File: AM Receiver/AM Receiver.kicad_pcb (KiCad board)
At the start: 2 copper layers, 88.8 x 40.2 mm, 74 parts, among them IC1 NE612AD, IC2 NE612AD, IC3 74HC74, IC4 TDA1072AT, IC5 74HTC4046, IC7 L78L05_SO8, P1 10k, P2 50k, P3 50k, Q1 MMBFJ310LT1G, Q2 MMBFJ310LT1G, Q3 BC547, Q4 BC547, Q5 BC557, U6 L78L08_SO8

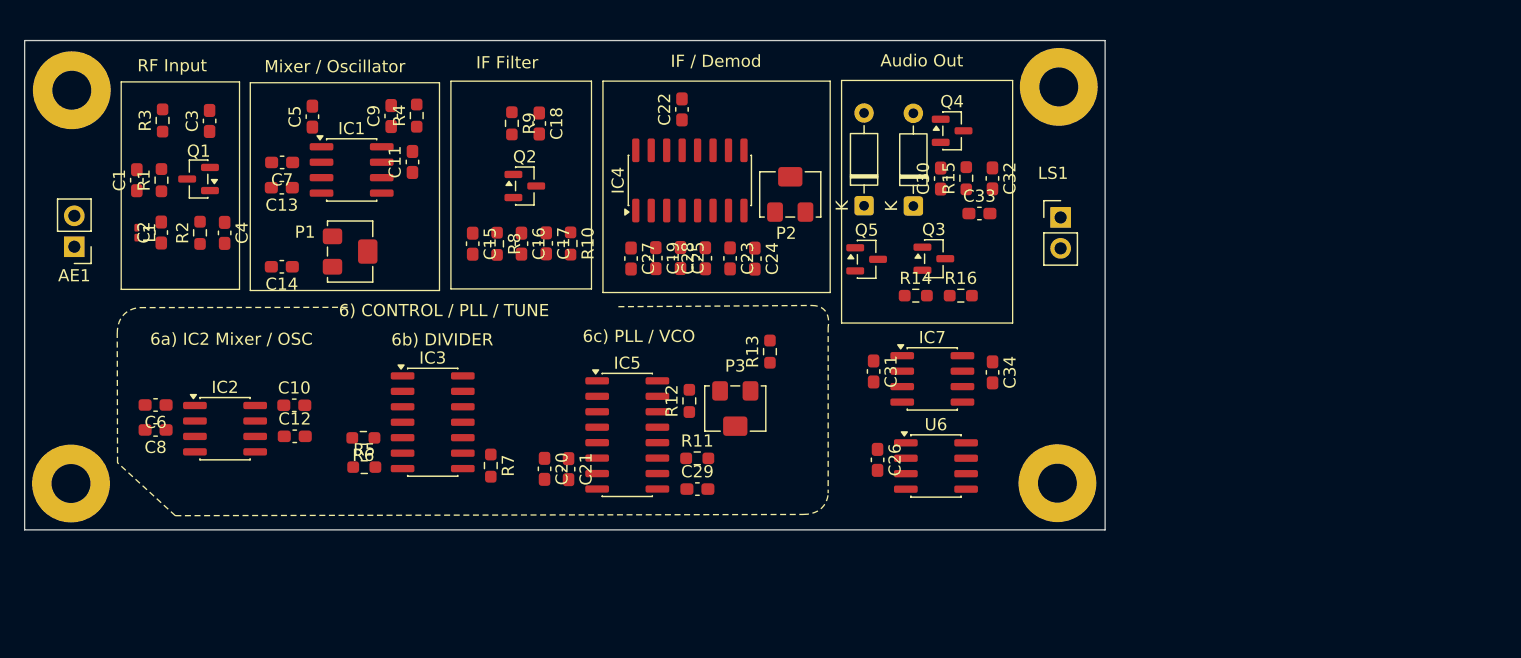
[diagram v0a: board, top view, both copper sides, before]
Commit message: Finished PCB design for AM Receiver and fixed all remaining errors
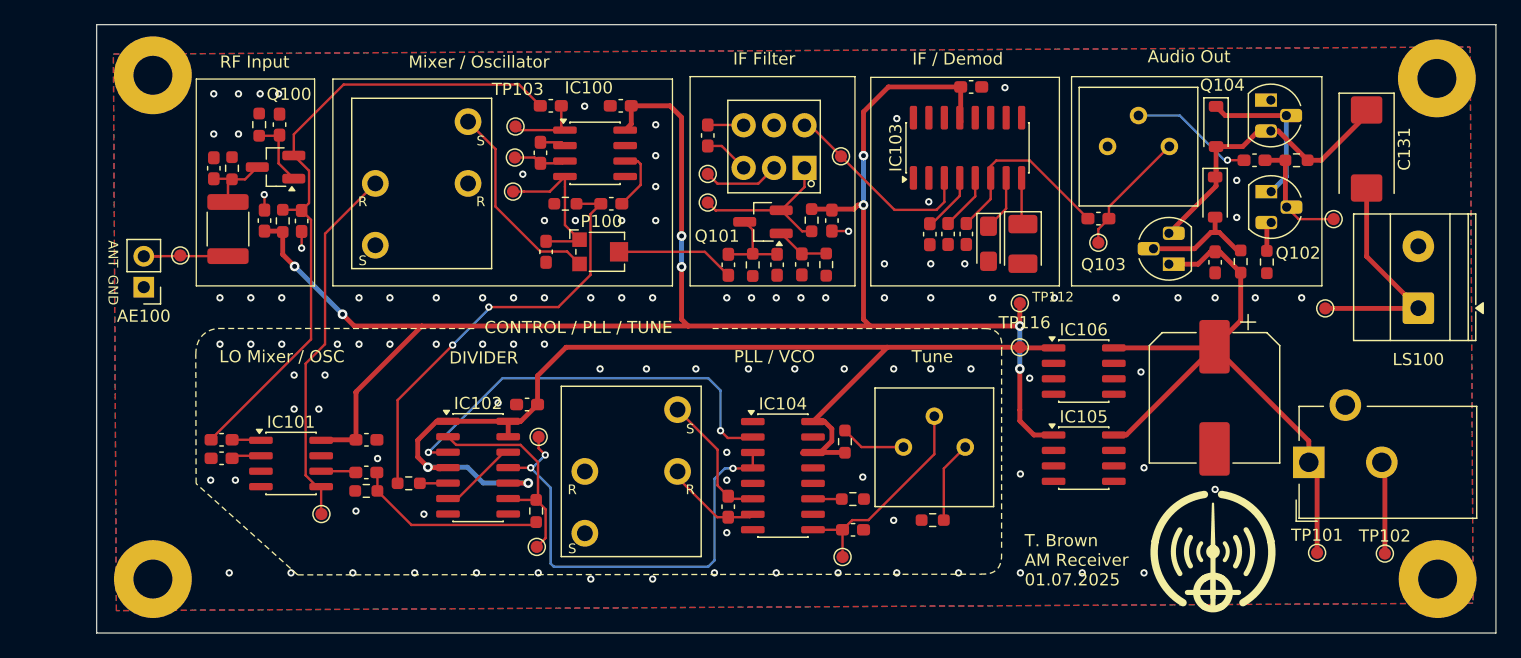
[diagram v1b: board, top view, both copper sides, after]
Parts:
- added AM_Radio_Logo: , AM_Radio:AM_Radio_logo, F.Cu at (184.2, 114.7)
- added FL100: SFZ455A, AM_Radio:SFZ455A, F.Cu at (148.2, 81.2)
- added J100: Barrel_Jack_Switch, Connector_BarrelJack:BarrelJack_CUI_PJ-102AH_Horizontal, F.Cu at (192.2, 107.2)
- added TP100: ANT_IN, TestPoint:TestPoint_Pad_D1.0mm, F.Cu at (99.4, 90.2)
- added TP101: TP_VIN, TestPoint:TestPoint_Pad_D1.0mm, F.Cu at (192.8, 114.6)
- added TP102: TP_GND, TestPoint:TestPoint_Pad_D1.0mm, F.Cu at (198.4, 114.7)
- added TP103: TP_MIXER_IN, TestPoint:TestPoint_Pad_D1.0mm, F.Cu at (127.0, 79.6)
- added TP104: TP_GND_RF, TestPoint:TestPoint_Pad_D1.0mm, F.Cu at (126.9, 82.1)
- added TP105: TP_RF_MIXER_OUT, TestPoint:TestPoint_Pad_D1.0mm, F.Cu at (126.8, 84.9)
- added TP106: TP_LO_MIXER_OUT, TestPoint:TestPoint_Pad_D1.0mm, F.Cu at (111.0, 111.4)
- added TP107: TP_IF_FILTER_IN, TestPoint:TestPoint_Pad_D1.0mm, F.Cu at (142.8, 85.8)
- added TP108: TP_DIV_OUT, TestPoint:TestPoint_Pad_D1.0mm, F.Cu at (128.7, 114.1)
- added TP109: TP_GND_IF, TestPoint:TestPoint_Pad_D1.0mm, F.Cu at (142.8, 83.5)
- added TP110: TP_IF_FILTER_OUT, TestPoint:TestPoint_Pad_D1.0mm, F.Cu at (153.7, 82.0)
- added TP111: TP_VCO_OUT, TestPoint:TestPoint_Pad_D1.0mm, F.Cu at (128.9, 105.1)
- added TP112: TP_8V, TestPoint:TestPoint_Pad_D1.0mm, F.Cu at (168.4, 94.1)
- added TP113: TP_AUDIO_DEMOD, TestPoint:TestPoint_Pad_D1.0mm, F.Cu at (174.9, 89.1)
- added TP114: TP_VCO_CTRL, TestPoint:TestPoint_Pad_D1.0mm, F.Cu at (153.8, 115.0)
- added TP115: TP_AUDIO_DRV, TestPoint:TestPoint_Pad_D1.0mm, F.Cu at (194.2, 87.2)
- added TP116: TP_5V, TestPoint:TestPoint_Pad_D1.0mm, F.Cu at (168.4, 97.7)
- added TP117: TP_SPK_OUT, TestPoint:TestPoint_Pad_D1.0mm, F.Cu at (193.5, 94.5)
- C113: renamed from C14; value 100p -> 7–100p; footprint Capacitor_SMD:C_0603_1608Metric_Pad1.08x0.95mm_HandSolder -> AM_Radio:Vishay_BFC280907015_Trimmer_7-100pF
- C120: renamed from C21; value 100p -> 7–100p; footprint Capacitor_SMD:C_0603_1608Metric_Pad1.08x0.95mm_HandSolder -> AM_Radio:Vishay_BFC280907015_Trimmer_7-100pF
- C122: renamed from C23; footprint Capacitor_SMD:C_0603_1608Metric_Pad1.08x0.95mm_HandSolder -> Capacitor_Tantalum_SMD:CP_EIA-3216-18_Kemet-A_HandSolder
- C123: renamed from C24; footprint Capacitor_SMD:C_0603_1608Metric_Pad1.08x0.95mm_HandSolder -> Capacitor_Tantalum_SMD:CP_EIA-3528-21_Kemet-B_HandSolder
- C131: renamed from C32; footprint Capacitor_SMD:C_0603_1608Metric_Pad1.08x0.95mm_HandSolder -> Capacitor_Tantalum_SMD:CP_EIA-7343-20_Kemet-V_HandSolder
- C132: renamed from C33; footprint Capacitor_SMD:C_0603_1608Metric_Pad1.08x0.95mm_HandSolder -> Capacitor_SMD:CP_Elec_10x10.5
- D100: renamed from D1; footprint Diode_THT:D_DO-35_SOD27_P7.62mm_Horizontal -> Diode_SMD:D_SOD-123
- D101: renamed from D2; footprint Diode_THT:D_DO-35_SOD27_P7.62mm_Horizontal -> Diode_SMD:D_SOD-123
- IC100: renamed from IC1; value NE612AD -> SA612AD
- IC101: renamed from IC2; value NE612AD -> SA612AD
- IC102: renamed from IC3; value 74HC74 -> 74HC74D
- IC104: renamed from IC5; value 74HTC4046 -> 74HCT4046AD
- L100: renamed from L1; footprint Inductor_SMD:L_0201_0603Metric_Pad0.64x0.40mm_HandSolder -> Inductor_SMD:L_1812_4532Metric_Pad1.30x3.40mm_HandSolder
- LS100: renamed from LS1; footprint Connector_PinHeader_2.54mm:PinHeader_1x02_P2.54mm_Vertical -> TerminalBlock_Phoenix:TerminalBlock_Phoenix_MKDS-1,5-2-5.08_1x02_P5.08mm_Horizontal
- P100: renamed from P1; footprint Potentiometer_SMD:Potentiometer_Bourns_3224W_Vertical -> Potentiometer_SMD:Potentiometer_Bourns_TC33X_Vertical
- P101: renamed from P2; footprint Potentiometer_SMD:Potentiometer_Bourns_3224W_Vertical -> Potentiometer_THT:Potentiometer_Bourns_3386P_Vertical
- P102: renamed from P3; footprint Potentiometer_SMD:Potentiometer_Bourns_3224W_Vertical -> Potentiometer_THT:Potentiometer_Bourns_3386P_Vertical
- Q100: renamed from Q1; value MMBFJ310LT1G -> MMBFJ310LT3G; footprint Package_TO_SOT_SMD:SOT-23 -> Package_TO_SOT_SMD:SOT-23_Handsoldering
- Q101: renamed from Q2; value MMBFJ310LT1G -> MMBFJ310LT3G; footprint Package_TO_SOT_SMD:SOT-23 -> Package_TO_SOT_SMD:SOT-23_Handsoldering
- Q102: renamed from Q3; footprint Package_TO_SOT_SMD:SOT-23 -> Package_TO_SOT_THT:TO-92_HandSolder
- Q103: renamed from Q4; footprint Package_TO_SOT_SMD:SOT-23 -> Package_TO_SOT_THT:TO-92_HandSolder
- Q104: renamed from Q5; footprint Package_TO_SOT_SMD:SOT-23 -> Package_TO_SOT_THT:TO-92_HandSolder
- moved Q104 35.7 mm to (189.0, 77.4), turned to -90 degrees
- moved R113 33.2 mm to (191.1, 82.4), turned to 180 degrees
- moved C127 32.5 mm to (174.9, 87.2), turned to 180 degrees
- moved H101 32.2 mm to (202.7, 116.8)
- moved P101 31.4 mm to (180.7, 81.2), turned to 90 degrees
- moved H102 31.1 mm to (202.7, 75.6)
- moved C131 30.8 mm to (196.9, 81.4)
- moved LS100 30.3 mm to (201.2, 94.5), turned to 90 degrees
- moved D101 29.7 mm to (184.5, 79.6), turned to -90 degrees
- moved C130 28.6 mm to (127.9, 102.4), turned to 180 degrees
- moved Q102 28.3 mm to (189.1, 84.9), turned to -90 degrees
- moved C126 27.6 mm to (164.0, 88.4)
- moved R108 25.9 mm to (151.3, 87.3)
- moved C129 25.8 mm to (187.7, 82.4), turned to 180 degrees
- moved R115 25.3 mm to (188.7, 90.7), turned to -90 degrees
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- renumbered AE1 to AE100, C1 to C100, C2 to C101, C3 to C102, C4 to C103, C5 to C104, C6 to C105, C7 to C106, C8 to C107, C9 to C108, C10 to C109, C11 to C110, C12 to C111, C13 to C112, C15 to C114, C16 to C115, C17 to C116, C18 to C117, C19 to C118, C20 to C119, C22 to C121, C25 to C124, C26 to C125, C27 to C126, C28 to C127, C29 to C128, C30 to C129, C31 to C130, C34 to C133, H1 to H100, H3 to H101, H2 to H102, H4 to H103, IC4 to IC103, U6 to IC105, IC7 to IC106, R1 to R100, R2 to R101, R3 to R102, R4 to R103, R5 to R104, R6 to R105, R7 to R106, R8 to R107, R9 to R108, R10 to R109, R11 to R110, R12 to R111, R13 to R112, R14 to R113, R15 to R114, R16 to R115
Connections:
- AE100 pad 1: Net-(AE1-A) -> GND
- AE100 pad 2: (no net) -> Net-(AE100-Pad2)
- C117 pad 1: Net-(C18-Pad1) -> Net-(C117-Pad1)
- C117 pad 2: Net-(Q2-D) -> Net-(C117-Pad2)
- IC103 pad 1: (no net) -> unconnected-(IC103-Pad1)
- IC103 pad 10: (no net) -> unconnected-(IC103-Pad10)
- IC103 pad 11: (no net) -> unconnected-(IC103-Pad11)
- IC103 pad 12: (no net) -> unconnected-(IC103-Pad12)
- IC103 pad 14: (no net) -> unconnected-(IC103-Pad14)
- IC103 pad 15: (no net) -> unconnected-(IC103-Pad15)
- IC103 pad 3: Net-(C18-Pad1) -> Net-(FL100-Pad6)
- IC103 pad 9: (no net) -> unconnected-(IC103-Pad9)
- L100 pad 2: Net-(AE1-A) -> Net-(AE100-Pad2)
- Q101 pad 2: Net-(Q2-D) -> Net-(Q101-D)
- R108 pad 2: Net-(Q2-D) -> Net-(Q101-D)
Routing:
- net +8V: track 0.00 -> 151.8 mm, vias 0 -> 8
- net +5V: track 0.00 -> 90.1 mm, vias 0 -> 2
- net +12V ...+15V: track 0.00 -> 54.2 mm
- net Net-(Q100-D): track 0.00 -> 53.8 mm
- net Net-(IC102B-C): track 0.00 -> 39.1 mm, vias 0 -> 3
- net Net-(C110-Pad2): track 0.00 -> 35.2 mm, vias 0 -> 2
- net Net-(IC102A-C): track 0.00 -> 34.9 mm, vias 0 -> 2
- net Net-(IC101-OUTB): track 0.00 -> 30.6 mm
- net Net-(D100-K): track 0.00 -> 23.4 mm
- net GND: track 0.00 -> 22.4 mm, vias 0 -> 107
- net Net-(C131-Pad2): track 0.00 -> 19.7 mm
- net Net-(IC102A-D): track 0.00 -> 18.2 mm
- net Net-(IC104-VCO_IN): track 0.00 -> 17.9 mm
- net Net-(C113-Pad1): track 0.00 -> 16.8 mm
- net Net-(C126-Pad1): track 0.00 -> 16.7 mm
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- added copper zone on B.Cu, net GND
- added copper zone on F.Cu, net GND
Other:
- board size 88.8 x 40.2 mm -> 115 x 50 mm
- board text added: "ANT"
- board text added: "CONTROL / PLL / TUNE"
- board text added: "DIVIDER"
- board text added: "GND"
- board text added: "LO Mixer / OSC"
- board text added: "PLL / VCO"
- board text added: "T. Brown AM Receiver 01.07.2025"
- board text added: "Tune"
- board text removed: "6) CONTROL / PLL / TUNE"
- board text removed: "6a) IC2 Mixer / OSC"
- board text removed: "6b) DIVIDER"
- board text removed: "6c) PLL / VCO"
